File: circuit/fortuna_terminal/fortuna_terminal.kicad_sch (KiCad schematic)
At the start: 14 parts

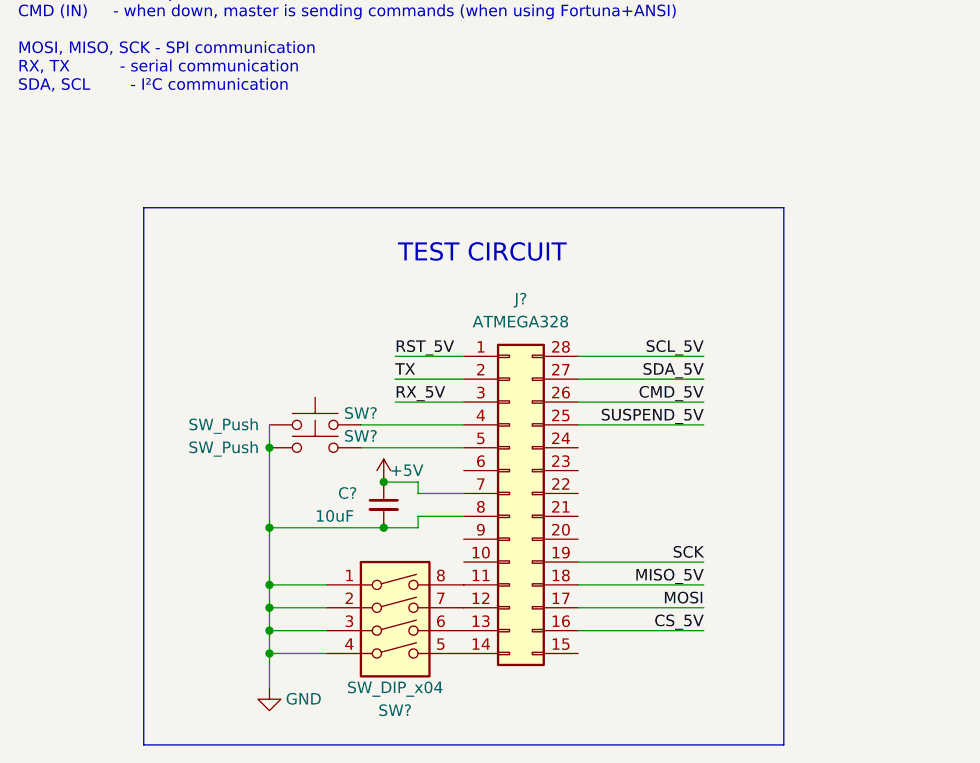
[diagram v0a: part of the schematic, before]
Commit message: .
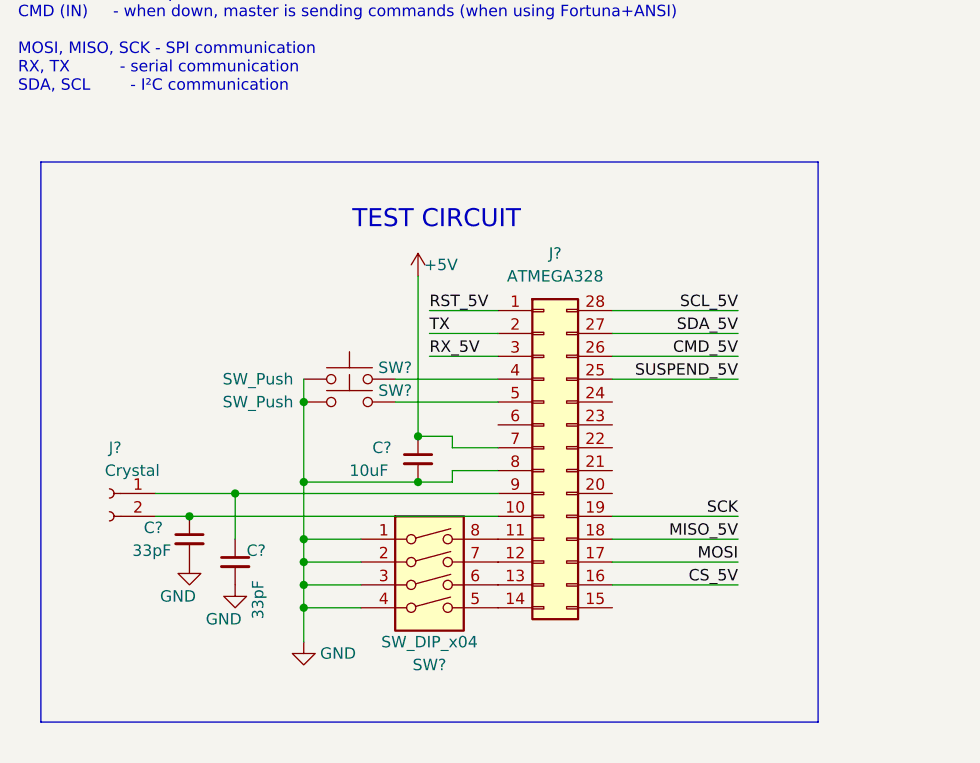
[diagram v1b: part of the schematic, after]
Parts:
- added C? (x2): 33pF, symbol Device:C_Small
- added J?: Crystal, symbol Connector:Conn_01x02_Female
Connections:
- net GND: now also C?.2, C?.2
- net at J?.10 (Pin_10): now also C?.1, J?.2 (Pin_2)
- net at J?.9 (Pin_9): now also C?.1, J?.1 (Pin_1)
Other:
- moved on the sheet: C?, J?, SW?
